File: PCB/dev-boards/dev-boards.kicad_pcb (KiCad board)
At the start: 2 copper layers, 160 x 152.4 mm, 4 parts, among them J1 Screw_Terminal_01x02, J2 SIM7600 Dev Board, U1 NUCLEO-F429ZI, U2 NUCLEO-F429ZI

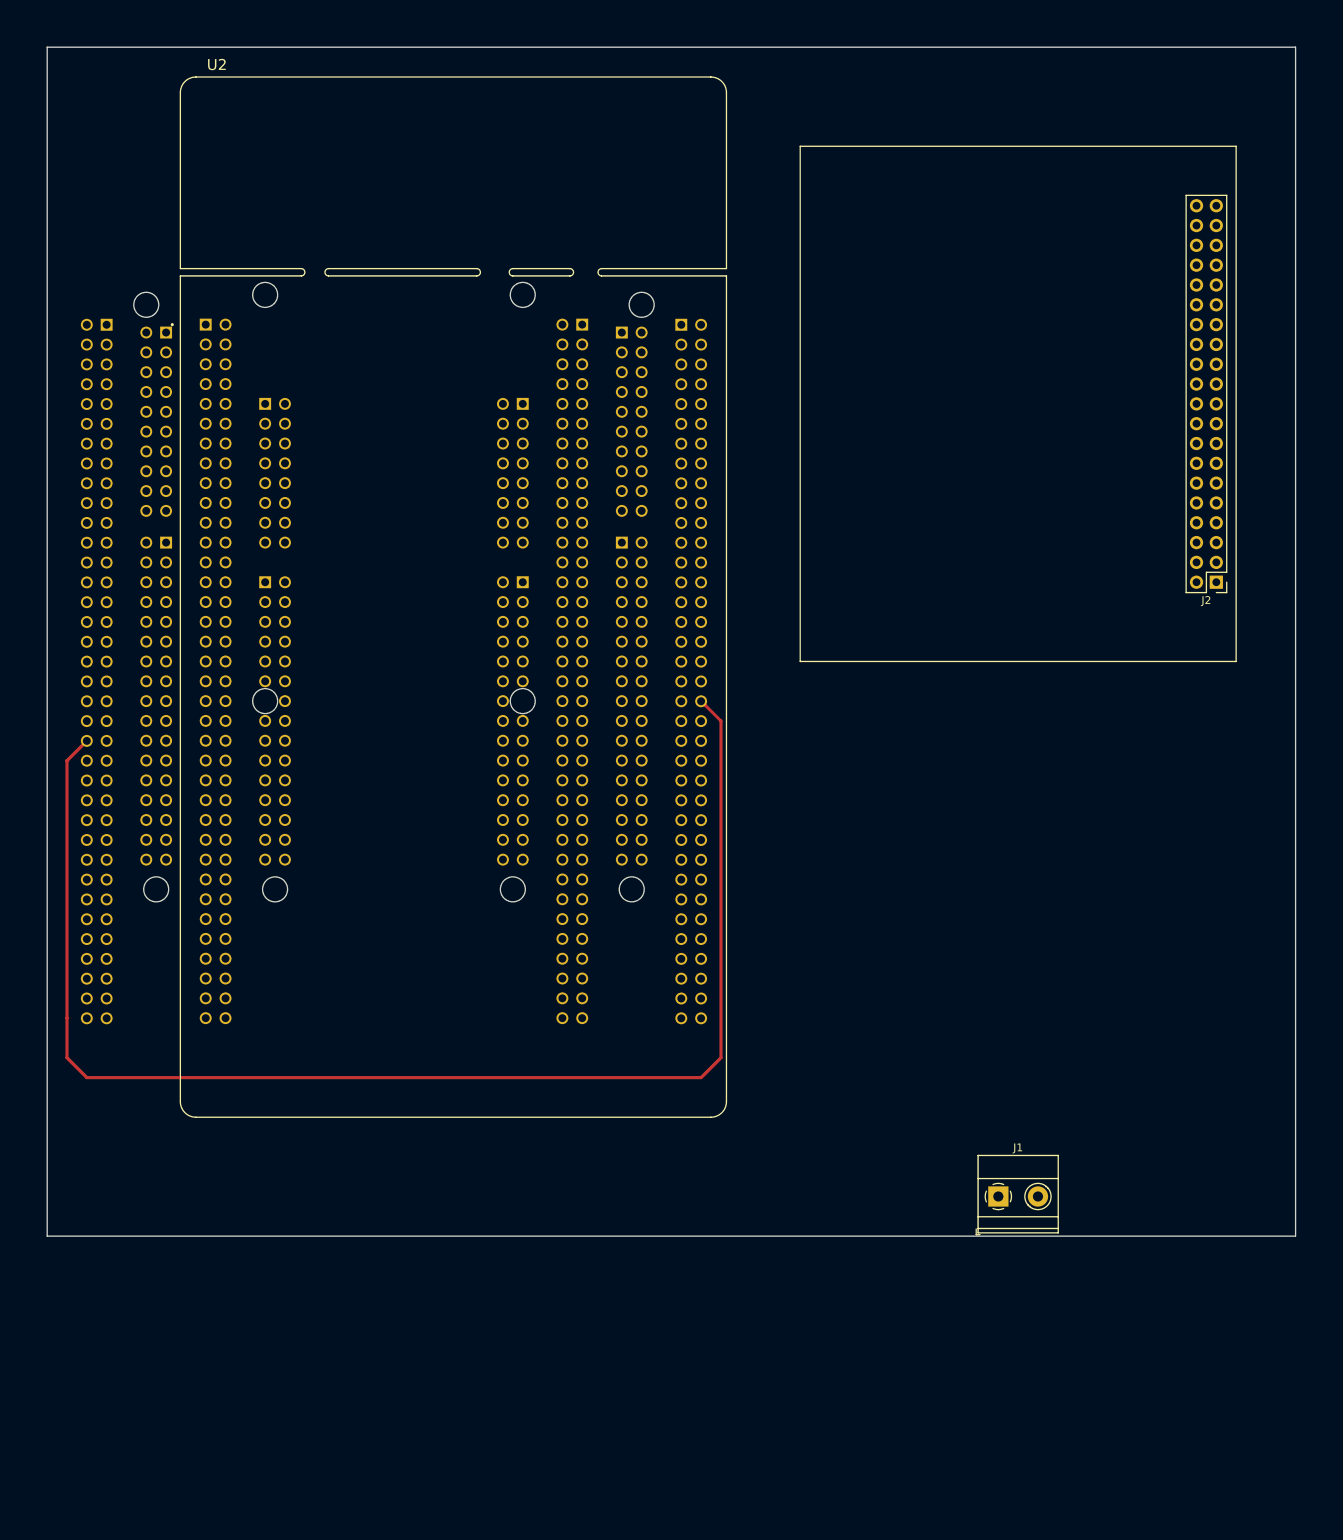
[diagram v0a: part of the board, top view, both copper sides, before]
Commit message: PCB board updates
Signed-off-by: Andrew Balmos <abalmos@purdue.edu>
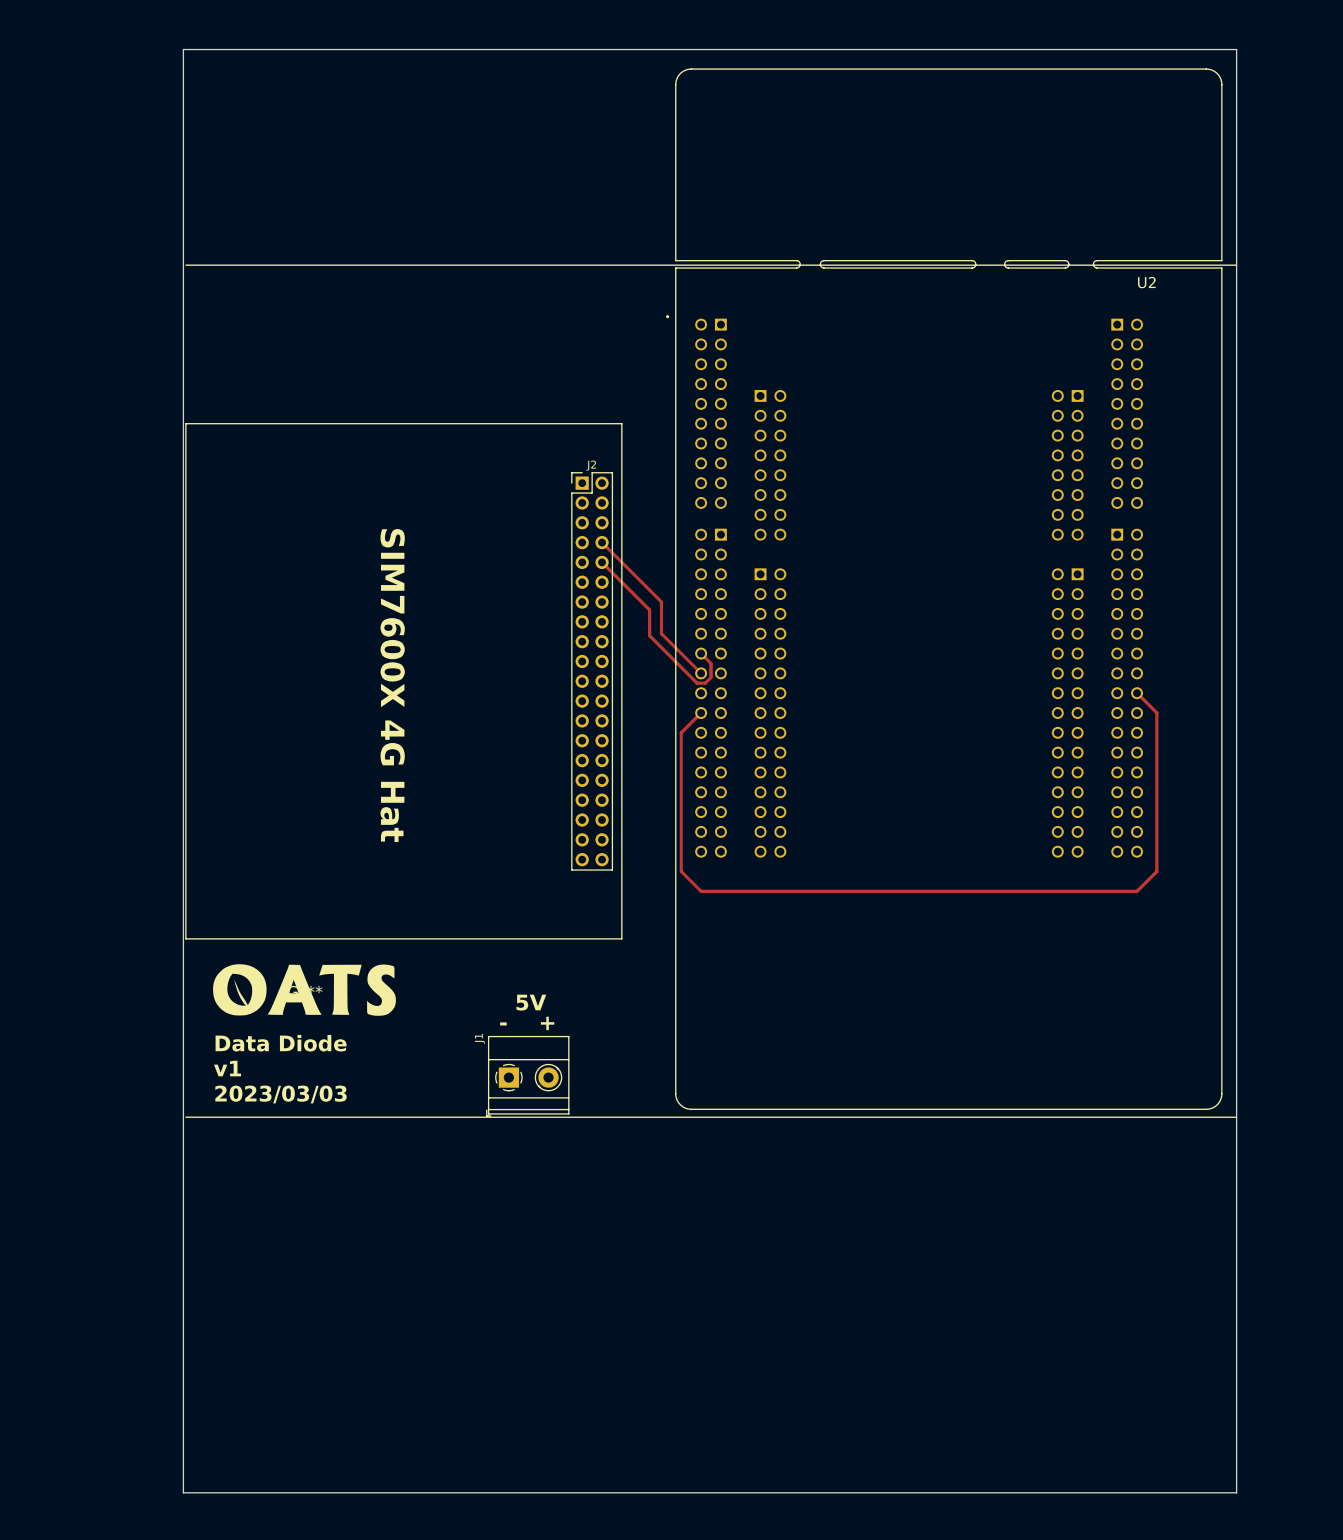
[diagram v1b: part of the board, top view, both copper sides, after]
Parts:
- added G***: LOGO, Local footprints:oats_logo, F.Cu at (35.6, 133.9)
- J1: value Screw_Terminal_01x02 -> 5V Input
- J2: value SIM7600 Dev Board -> SIM7600 Cell Header
- moved J2 82.3 mm to (71.1, 68.6), turned to 0 degrees
- moved U1 71.1 mm to (110.5, 82.2)
- moved J1 64.6 mm to (61.7, 144.8)
- moved U2 63.5 mm to (118.1, 82.2)
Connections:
- J2 pad 10: unconnected-(J2-Pin_10-Pad10) -> /M_RX_TX
- J2 pad 13: GND -> unconnected-(J2-Pin_13-Pad13)
- J2 pad 14: unconnected-(J2-Pin_14-Pad14) -> GND
- J2 pad 2: unconnected-(J2-Pin_2-Pad2) -> +5V
- J2 pad 24: GND -> unconnected-(J2-Pin_24-Pad24)
- J2 pad 25: unconnected-(J2-Pin_25-Pad25) -> GND
- J2 pad 26: GND -> unconnected-(J2-Pin_26-Pad26)
- J2 pad 30: unconnected-(J2-Pin_30-Pad30) -> GND
- J2 pad 31: GND -> unconnected-(J2-Pin_31-Pad31)
- J2 pad 38: GND -> unconnected-(J2-Pin_38-Pad38)
- J2 pad 39: +5V -> GND
- J2 pad 4: unconnected-(J2-Pin_4-Pad4) -> +5V
- J2 pad 40: +5V -> unconnected-(J2-Pin_40-Pad40)
- J2 pad 5: GND -> unconnected-(J2-Pin_5-Pad5)
- J2 pad 6: unconnected-(J2-Pin_6-Pad6) -> GND
- J2 pad 8: unconnected-(J2-Pin_8-Pad8) -> /M_TX_RX
- J2 pad 9: unconnected-(J2-Pin_9-Pad9) -> GND
- U1 pad CN10_14: unconnected-(U1F-D1/USART_A_TX-PadCN10_14) -> /M_RX_TX
- U1 pad CN10_16: unconnected-(U1F-D0/USART_A_RX-PadCN10_16) -> /M_TX_RX
- U1 pad CN10_20: unconnected-(U1F-D41/TIMER_A_ETR-PadCN10_20) -> /TSC Side Sheet/D_TX
- U2 pad CN10_18: unconnected-(U2F-D42/TIMER_A_PWM1N-PadCN10_18) -> /TSC Side Sheet/D_TX
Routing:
- net /TSC Side Sheet/D_TX: track 174.4 -> 108.3 mm
- net /M_RX_TX: track 0.00 -> 26.2 mm
- net /M_TX_RX: track 0.00 -> 22.0 mm
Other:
- board size 160 x 152.4 mm -> 135 x 185 mm
- rule pad_to_mask_clearance: 0 -> 0.05
- board text added: "+"
- board text added: "-"
- board text added: "5V"
- board text added: "Data Diode v1 2023/03/03"
- board text added: "SIM7600X 4G Hat"
- board text added: "TSC Nucleo-144"
- board text added: "World Side Nucleo-144"

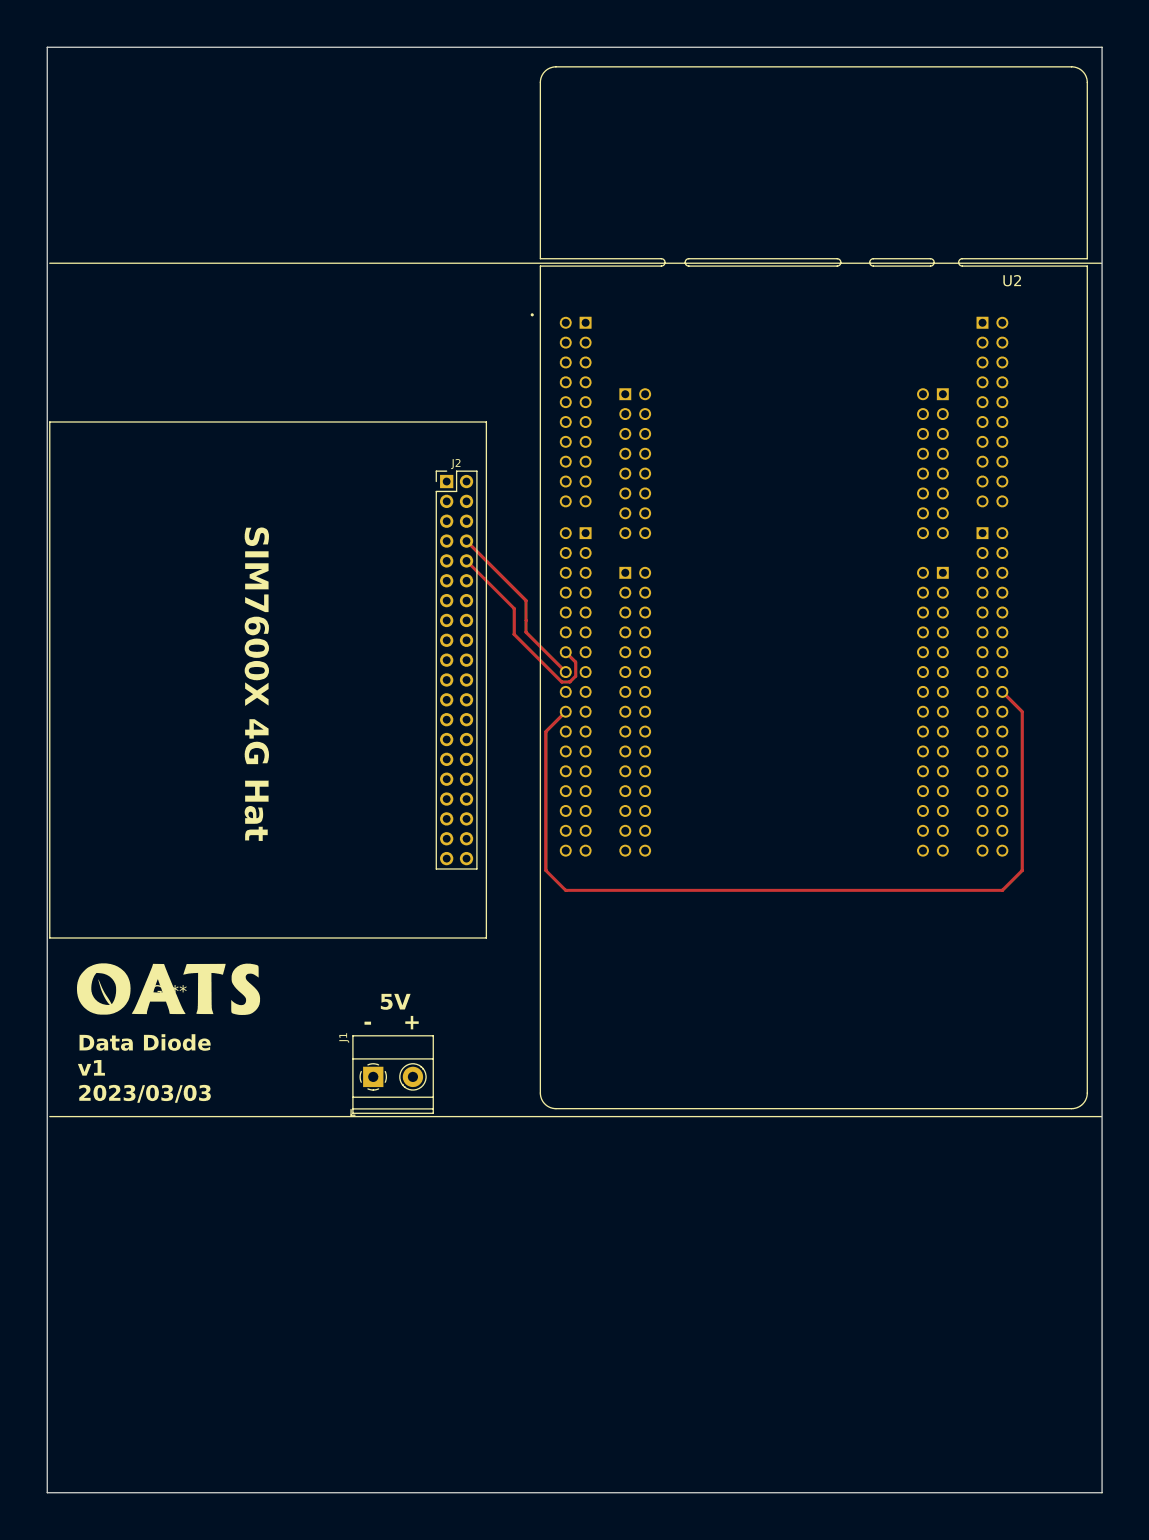
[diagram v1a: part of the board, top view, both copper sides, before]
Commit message: Update PCB for JLCPCB
Signed-off-by: Andrew Balmos <abalmos@purdue.edu>
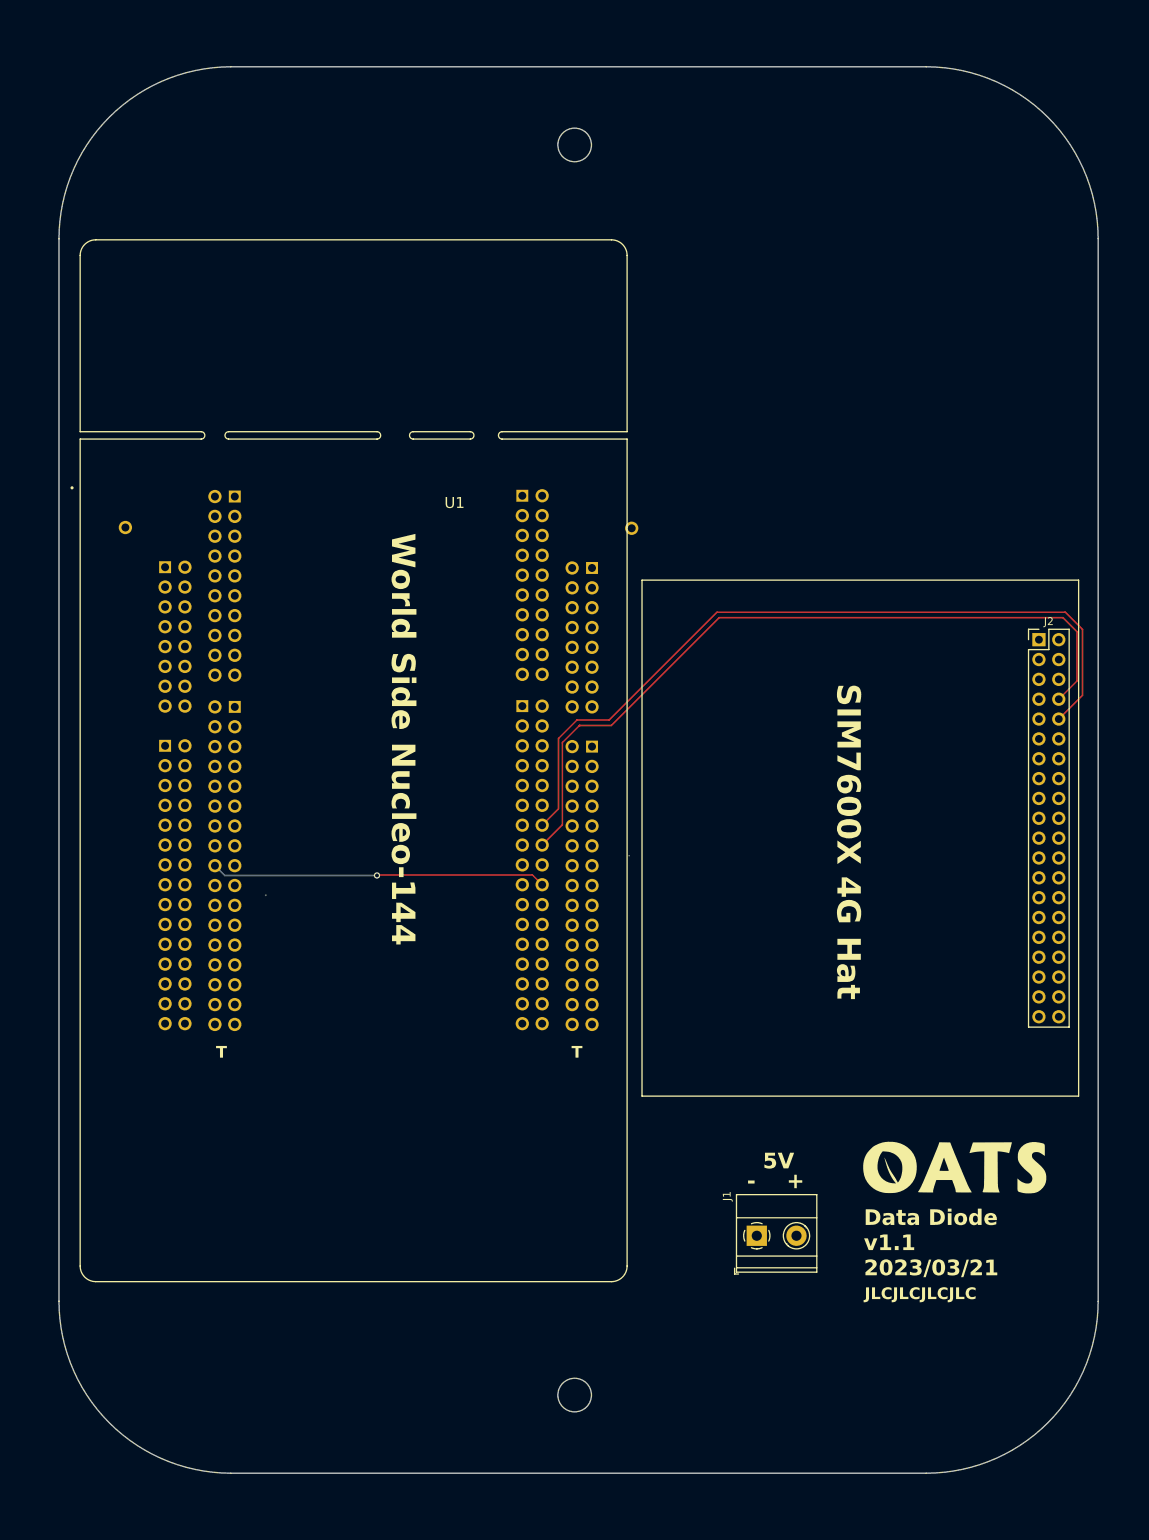
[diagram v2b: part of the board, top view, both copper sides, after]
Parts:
- removed G***: LOGO, Local footprints:oats_logo
- added H1: MountingHole, MountingHole:MountingHole_4.3mm_M4, F.Cu at (87.5, 25.5)
- added H2: MountingHole, MountingHole:MountingHole_4.3mm_M4, F.Cu at (87.5, 185.5)
- added N1: Housing, Local footprints:oats_logo, F.Cu at (136.2, 156.7)
- U1: moved to F.Cu
- U2: moved to B.Cu
- moved J2 78.5 mm to (146.9, 88.8)
- moved U2 57.0 mm to (65.6, 104.4), turned to 180 degrees
- moved U1 55.9 mm to (59.2, 104.3), turned to 0 degrees
- moved J1 53.1 mm to (110.8, 165.1)
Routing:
- net /M_TX_RX: track 22.0 -> 97.1 mm
- net /M_RX_TX: track 26.2 -> 99.4 mm
- net /TSC Side Sheet/D_TX: track 108.3 -> 42.9 mm, vias 0 -> 1
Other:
- board size 135 x 185 mm -> 133 x 180 mm
- board text added: "B"
- board text added: "Data Diode v1.1 2023/03/21"
- board text added: "JLCJLCJLCJLC"
- board text added: "T"
- board text removed: "Data Diode v1 2023/03/03"
